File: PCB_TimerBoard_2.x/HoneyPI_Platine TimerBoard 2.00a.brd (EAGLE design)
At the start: 63.5 x 32.7 mm, 17 parts, among them Q3 IRF9540

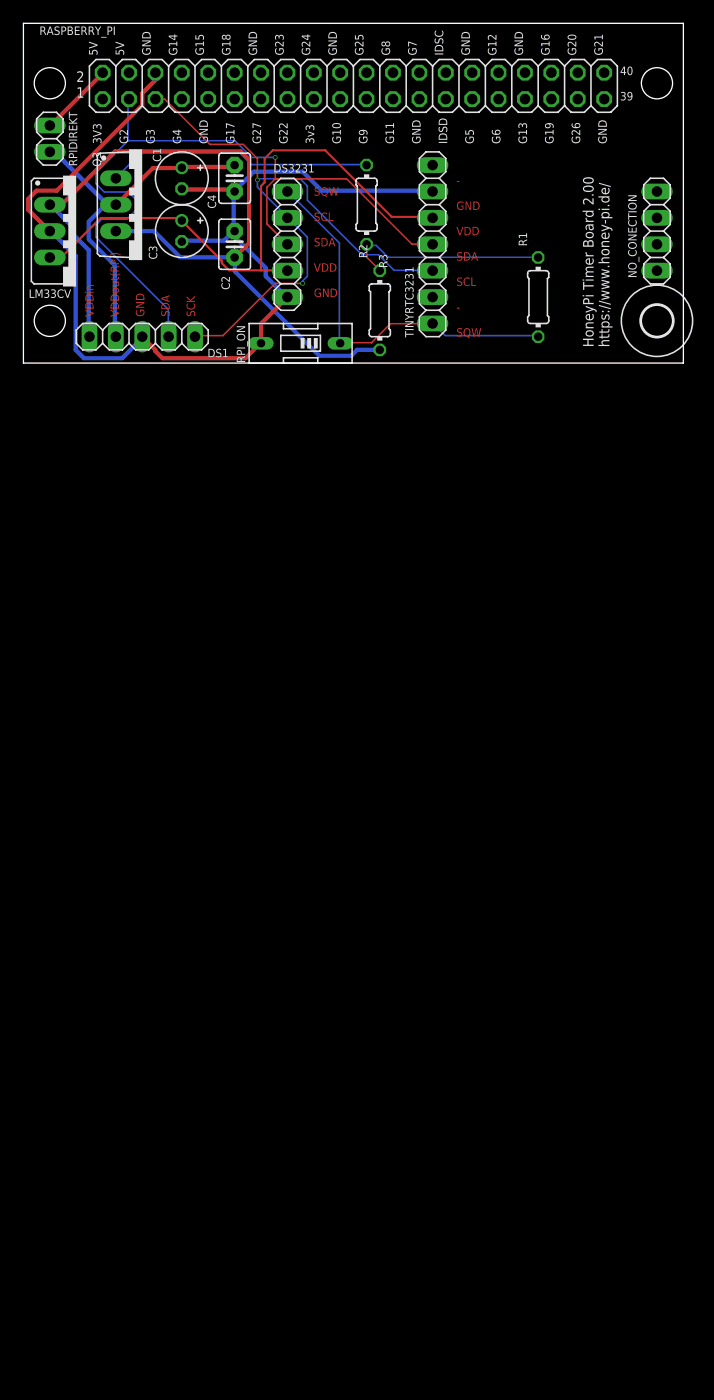
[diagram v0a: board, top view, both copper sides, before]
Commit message: Updates, updates....
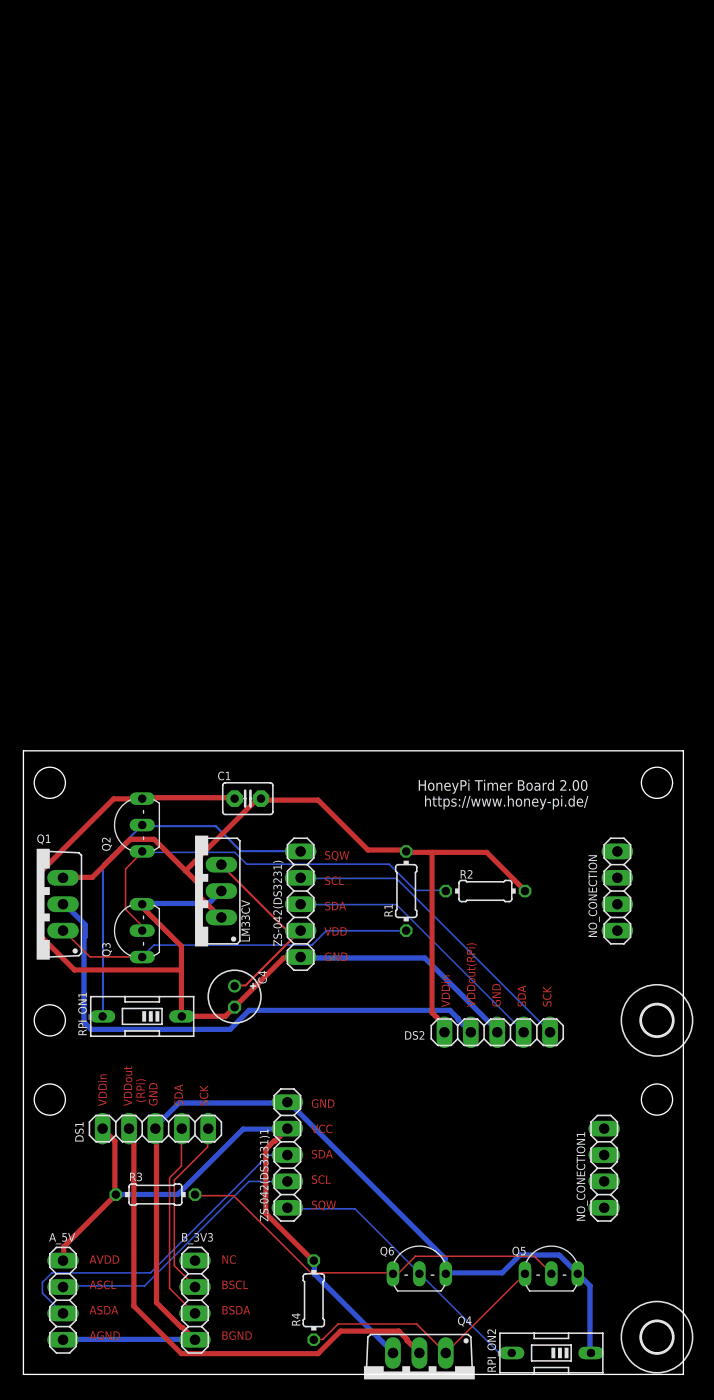
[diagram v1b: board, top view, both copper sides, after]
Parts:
- removed C2: 0,1µF, capacitor-wima:C2.5-3
- removed C3: 10µF, rcl:E2-5
- removed DS3231: (no value), pinhead:1X05
- removed RASPBERRY_PI: (no value), pinhead:2X20
- removed RPIDIREKT: (no value), pinhead:1X02
- removed RPI_ON: (no value), special:EDG-01
- removed TINYRTC3231: (no value), pinhead:1X07
- added A_5V, B_3V3, NO_CONECTION1: (no value), pinhead:1X04
- added DS2, ZS-042(DS3231), ZS-042(DS3231)1: (no value), pinhead:1X05
- added Q1, Q4: NDP6020P, transistor-power:TO220BV
- added Q2, Q5, Q6: BC547, transistor-npn:TO92-EBC
- added R4: 10k, rcl:0204/7
- added RPI_ON1, RPI_ON2: (no value), special:EDG-01
- added U$1: (no value), holes:3,0
- C1: value 100µF -> 0,1µF; device rcl:E2-5 -> capacitor-wima:C2.5-3
- C4: value 0,1µF -> 10µF; device capacitor-wima:C2.5-3 -> rcl:E2-5
- Q3: value IRF9540 -> BC547; device transistor-power:TO220BV -> transistor-npn:TO92-EBC
- R1: value 2,2KOhm -> 10k
- R2: value 10KOhm -> 10k
- R3: value 220Ohm -> 10k
- moved R3 97.4 mm to (12.7, -12.7), turned to 0 degrees
- moved C4 78.7 mm to (20.3, 6.35), turned to 270 degrees
- moved DS1 76.2 mm to (12.7, -6.35)
- moved Q3 69.9 mm to (10.2, 12.7), turned to 90 degrees
- moved U$7 67.3 mm to (61.0, 4.06)
- moved LM33CV 64.5 mm to (16.5, 16.5), turned to 90 degrees
- moved NO_CONECTION 63.6 mm to (57.1, 16.5)
- moved C1 60.0 mm to (21.6, 25.4), turned to 0 degrees
- moved R1 58.5 mm to (36.8, 16.5), turned to 90 degrees
- moved R2 56.8 mm to (44.5, 16.5), turned to 180 degrees
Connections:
- removed net 3V3_PIN1: RASPBERRY_PI.1
- removed net 5V_PIN2: RASPBERRY_PI.2, RPIDIREKT.1
- removed net BME_SCL/SCK_PIN5: DS1.5, DS3231.2, RASPBERRY_PI.5, TINYRTC3231.3
- removed net BME_SDI/SDA_PIN3: DS1.4, DS3231.3, RASPBERRY_PI.3, TINYRTC3231.4
- removed net GND2: C1.-, C2.1, C3.-, C4.1, DS1.3, DS3231.5, LM33CV.2, RASPBERRY_PI.6, RPI_ON.2, TINYRTC3231.6
- removed net N$9: R1.1, R2.1, R3.1
- removed net V_IN: C2.2, DS1.1, LM33CV.1, Q3.S, R2.2
- removed net V_OUT: C1.+, C4.2, DS1.2, Q3.D, RPIDIREKT.2
- new net ALARM_SQW_2: Q2.B, RPI_ON1.2, ZS-042(DS3231).1
- new net GND_1: A_5V.4, B_3V3.4, DS1.3, Q5.E, Q6.E, RPI_ON2.1, ZS-042(DS3231)1.5
- new net GND_2: C1.1, C4.-, DS2.3, LM33CV.2, Q2.E, Q3.E, RPI_ON1.1, ZS-042(DS3231).5
- new net N$1: Q4.G, Q5.C, R4.1
- new net N$5: Q1.G, Q3.C, R1.1
- new net N$6: Q2.C, Q3.B, R2.2
- new net N$7: A_5V.3, ZS-042(DS3231)1.3
- new net N$8: A_5V.2, ZS-042(DS3231)1.2
- new net SCL/SCK_PIN5_1: B_3V3.2, DS1.5
- new net SCL/SCK_PIN5_2: DS2.5, ZS-042(DS3231).2
- new net SDI/SDA_PIN3_1: B_3V3.3, DS1.4
- new net SDI/SDA_PIN3_2: DS2.4, ZS-042(DS3231).3
- new net V_IN_5V_1: A_5V.1, DS1.1, Q4.S, R3.1, R4.2, ZS-042(DS3231)1.4
- new net V_IN_5V_2: C1.2, DS2.1, LM33CV.1, Q1.S, R1.2, R2.1
- new net V_OUT_5V_1: DS1.2, Q4.D
- new net V_OUT_5V_2: DS2.2, Q1.D
- net ALARM_SQW: now also Q6.B, RPI_ON2.2, ZS-042(DS3231)1.1; no longer DS3231.1, R1.2, RPI_ON.1, TINYRTC3231.1
- net N$3: now also Q5.B, Q6.C; no longer Q3.G
- net V_LF33CV: now also C4.+, ZS-042(DS3231).4; no longer C3.+, DS3231.4, TINYRTC3231.5
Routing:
- net GND2: track 104.8 -> 0.00 mm
- net GND_2: track 0.00 -> 99.1 mm
- net GND_1: track 0.00 -> 93.8 mm
- net V_IN_5V_2: track 0.00 -> 77.6 mm
- net V_IN: track 77.3 -> 0.00 mm
- net BME_SDI/SDA_PIN3: track 75.2 -> 0.00 mm, vias 1 -> 0
- net V_IN_5V_1: track 0.00 -> 62.2 mm
- net BME_SCL/SCK_PIN5: track 60.2 -> 0.00 mm, vias 2 -> 0
- net V_OUT_5V_2: track 0.00 -> 51.6 mm
- net V_OUT_5V_1: track 0.00 -> 48.5 mm
- net N$6: track 0.00 -> 39.8 mm
- net V_LF33CV: track 56.8 -> 19.3 mm
- net V_OUT: track 36.9 -> 0.00 mm
- net ALARM_SQW_2: track 0.00 -> 36.4 mm
- net N$5: track 0.00 -> 35.1 mm
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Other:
- board size 63.5 x 32.7 mm -> 63.5 x 60 mm
- board text added: "AVDD ASCL ASDA AGND"
- board text added: "GND VCC SDA SCL SQW"
- board text added: "NC BSCL BSDA BGND"
- board text added: "VDDin VDDout (RPi) GND SDA SCK"
- board text removed: "- GND VDD SDA SCL - SQW"
- board text removed: "2 1"
- board text removed: "3V3 G2 G3 G4 GND G17 G27 G22 3v3 G10 G9 G11 GND IDSD G5 G6 G13 G19 G26 GND"
- board text removed: "40 39"
- board text removed: "5V 5V GND G14 G15 G18 GND G23 G24 GND G25 G8 G7 IDSC GND G12 GND G16 G20 G21"
